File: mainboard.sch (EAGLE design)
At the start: 75 parts, among them J1 POWER_JACKPTH_LOCK, T1 SINGLE_NCHAN_FET, T10 SINGLE_NCHAN_FET, T2 MOSFET_PCHAN_20A, T3 SINGLE_NCHAN_FET, T4 MOSFET_PCHAN_20A, T5 SINGLE_NCHAN_FET, T6 MOSFET_PCHAN_20A, T7 MOSFET_PCHAN_20A, T8 SINGLE_NCHAN_FET, T9 MOSFET_PCHAN_20A, U1 MURATA_REG_OKL-T3-W12, U2 TEENSY_3.0+4, U3 RFM23BP, U4 HMC5883LSMD, U5 ITG-3200, U7 CURRENT_MAX4372, U8 CURRENT_MAX4372

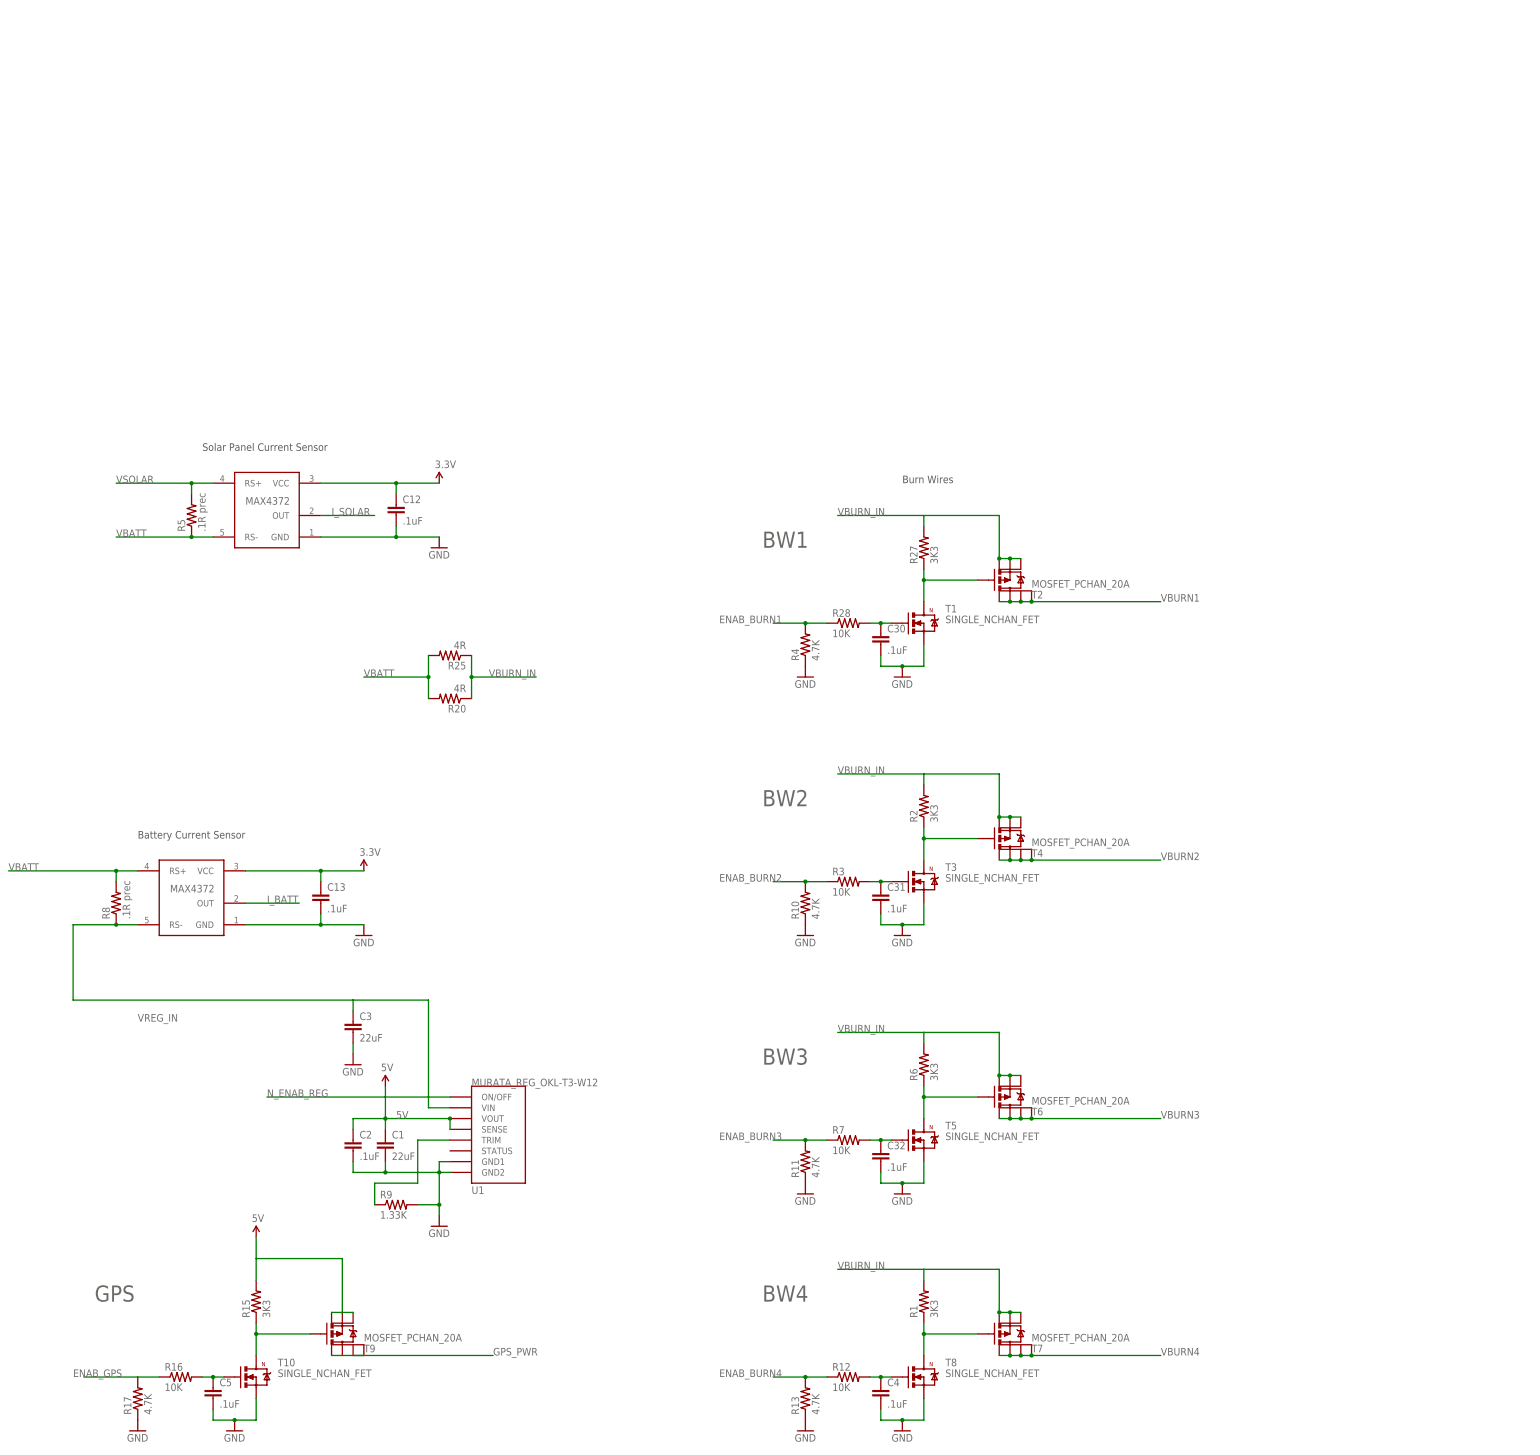
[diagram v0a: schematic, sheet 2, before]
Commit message: Schematic clean-up
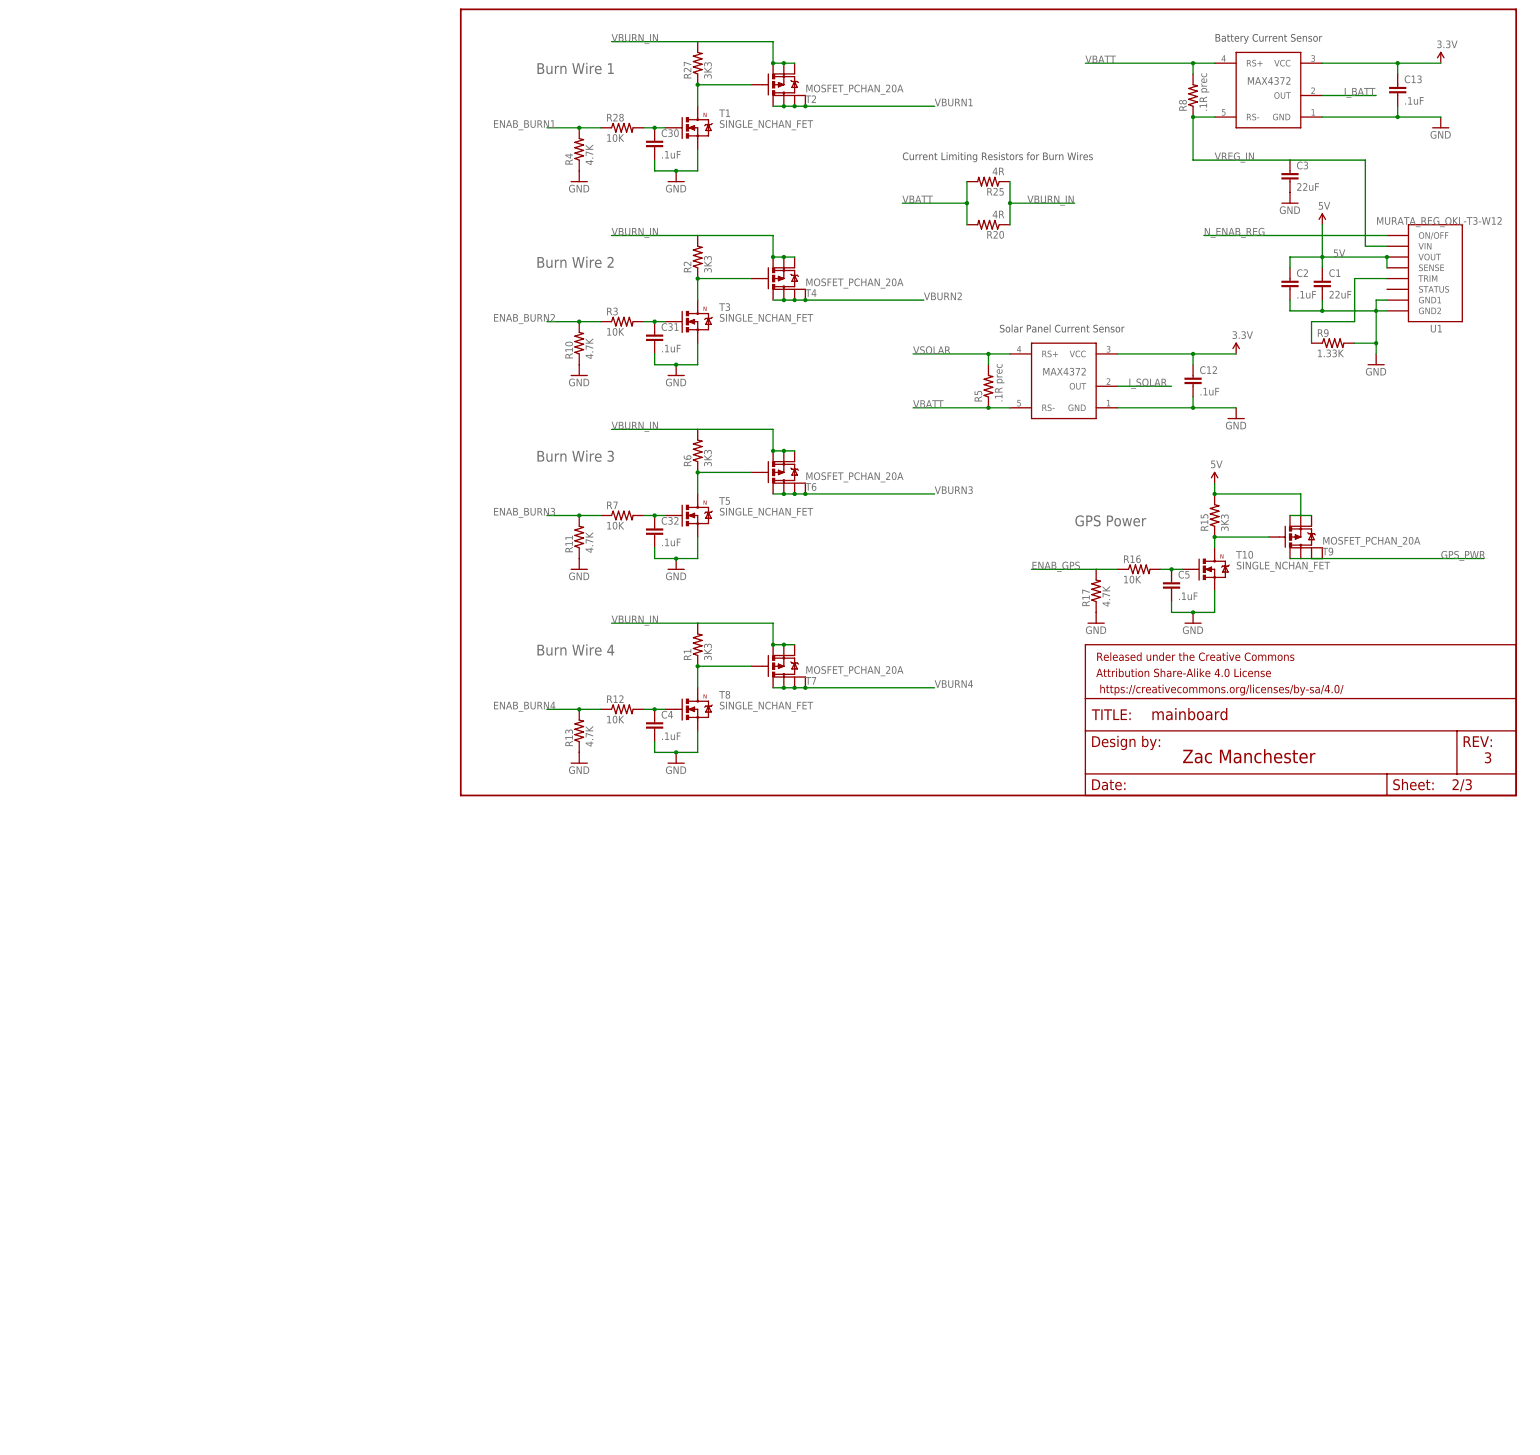
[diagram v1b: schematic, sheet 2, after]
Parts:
- added FRAME1, FRAME2, FRAME3: FRAME-LETTER, SparkFun-Aesthetics:FRAME-LETTER
- X1: device pel_molex:CONN_5-1-53398 -> pel_molex:CONN_5-1-53261
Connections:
- net N$11: now also S3.1; no longer S3.3
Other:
- note added: "3"
- note added: "Burn Wire 1"
- note added: "Burn Wire 2"
- note added: "Burn Wire 3"
- note added: "Burn Wire 4"
- note added: "Current Limiting Resistors for Burn Wires"
- note added: "GPS Power"
- note added: "Piksi GPS Connector"
- note added: "Zac Manchester"
- note removed: "BW1"
- note removed: "BW2"
- note removed: "BW3"
- note removed: "BW4"
- note removed: "Burn Wires"
- note removed: "GPS"
- moved on the sheet: C1, C12, C13, C14, C15, C16, C17, C18, C19, C2, C20, C3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
